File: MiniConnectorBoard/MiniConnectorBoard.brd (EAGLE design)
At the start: 31.1 x 68.6 mm, 4 parts

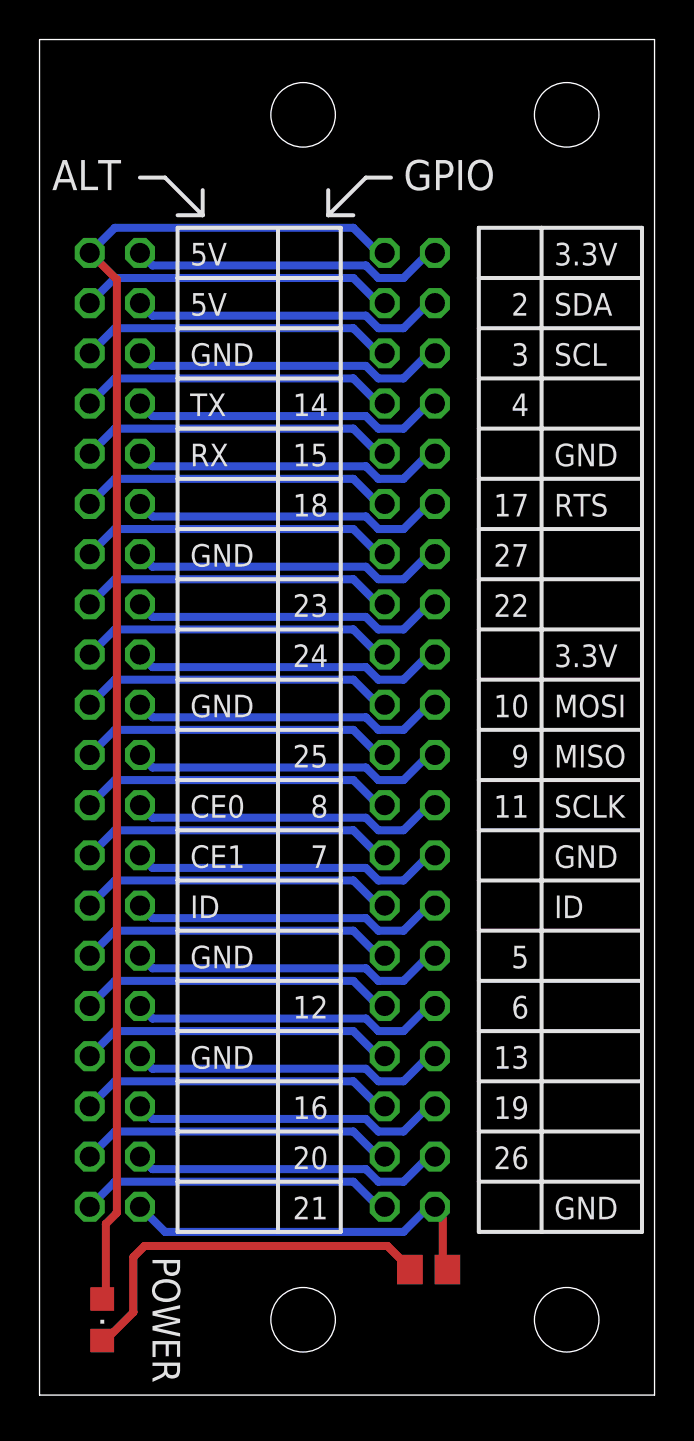
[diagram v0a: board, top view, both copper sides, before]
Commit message: MiniConnectorBoard - first cut
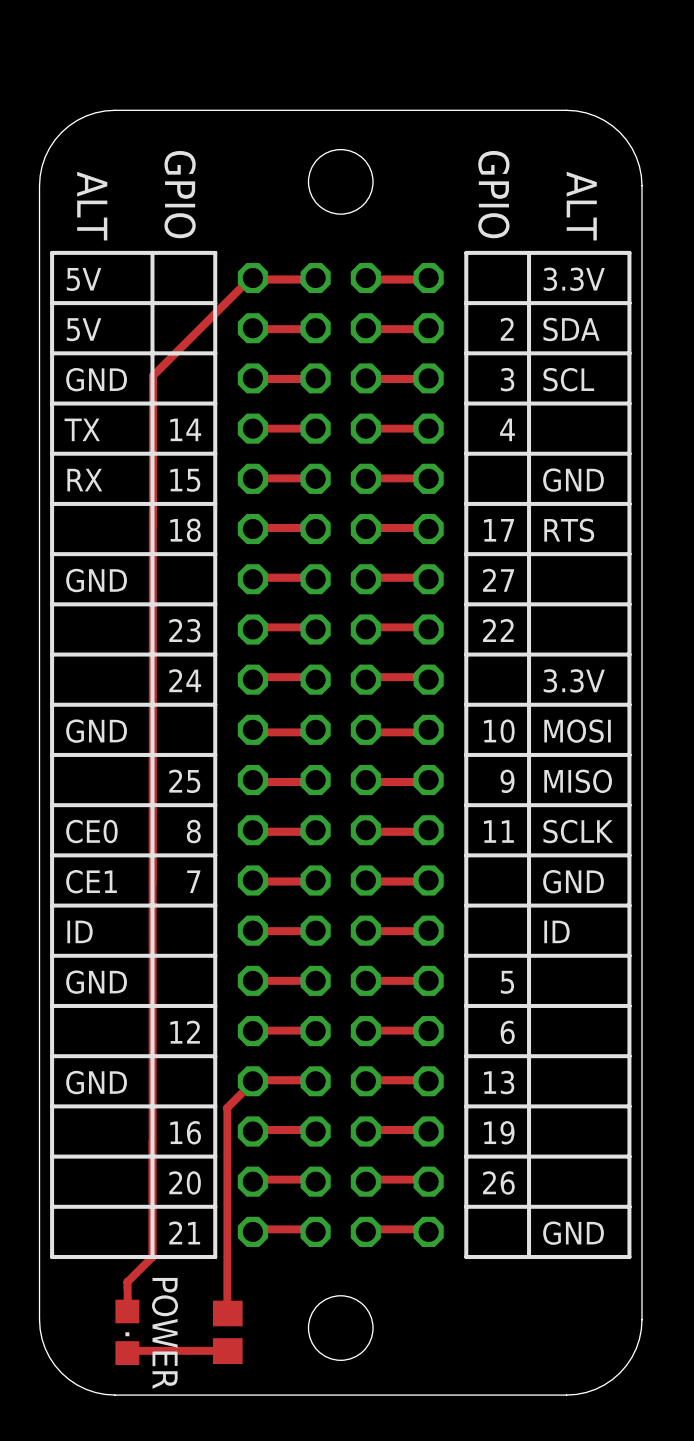
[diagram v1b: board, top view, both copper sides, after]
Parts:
- added JP3: NONE, MiniConnectorBoard:1X20
- JP2: device HeaderConnectorBoard:2X20 -> MiniConnectorBoard:1X20
- moved R1 10.6 mm to (9.53, 3.17), turned to 270 degrees
- moved JP2 8.35 mm to (12.1, 32.4)
- moved JP1 3.72 mm to (15.2, 32.4)
- moved LED1 1.42 mm to (4.45, 3.17)
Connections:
- net 10/MOSI: now also JP3.10; no longer JP2.20
- net 11/CLK: now also JP3.12; no longer JP2.24
- net 12: now also JP2.16; no longer JP2.31
- net 13: now also JP3.17; no longer JP2.34
- net 14/TX: now also JP2.4; no longer JP2.7
- net 15/RX: now also JP2.5; no longer JP2.9
- net 16: now also JP2.18; no longer JP2.35
- net 17/RTS: now also JP3.6; no longer JP2.12
- net 18: now also JP2.6; no longer JP2.11
- net 19: now also JP3.18; no longer JP2.36
- net 2/SDA: now also JP3.2; no longer JP2.4
- net 20: now also JP2.19; no longer JP2.37
- net 21: now also JP2.20; no longer JP2.39
- net 22: now also JP3.8; no longer JP2.16
- net 23: now also JP2.8; no longer JP2.15
- net 24: now also JP2.9; no longer JP2.17
- net 25: now also JP2.11; no longer JP2.21
- net 26: now also JP3.19; no longer JP2.38
- net 27: now also JP3.7; no longer JP2.14
- net 3.3V_1: now also JP3.1; no longer JP2.2
- net 3.3V_2: now also JP3.9; no longer JP2.18
- net 3/SCL: now also JP3.3; no longer JP2.6
- net 4: now also JP3.4; no longer JP2.8
- net 5: now also JP3.15; no longer JP2.30
- net 5V_1: now also JP2.2; no longer JP2.3
- net 6: now also JP3.16; no longer JP2.32
- net 7/CE1: now also JP2.13; no longer JP2.25
- net 8/CE0: now also JP2.12; no longer JP2.23
- net 9/MISO: now also JP3.11; no longer JP2.22
- net GND: now also JP3.5; no longer JP2.10
- net GND2: now also JP3.13; no longer JP2.26
- net GND3: now also JP2.10; no longer JP2.19
- net GND4: now also JP2.7; no longer JP2.13
- net GND5: now also JP2.3; no longer JP2.5
- net GND6: now also JP3.20; no longer JP2.40, R1.1
- net GND7: now also JP2.17, R1.1; no longer JP2.33
- net GND8: now also JP2.15; no longer JP2.29
- net ID1: now also JP3.14; no longer JP2.28
- net ID2: now also JP2.14; no longer JP2.27
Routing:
- net GND6: track 19.5 -> 3.26 mm
- net N$1: track 19.7 -> 5.17 mm
- net 5: track 16.0 -> 3.17 mm
- net 14/TX: track 16.0 -> 3.18 mm
- net 4: track 16.0 -> 3.17 mm
- net GND8: track 16.0 -> 3.18 mm
- net GND: track 16.0 -> 3.18 mm
- net ID1: track 16.0 -> 3.18 mm
- net 6: track 16.0 -> 3.18 mm
- net 3/SCL: track 16.0 -> 3.18 mm
- net 17/RTS: track 16.0 -> 3.19 mm
- net GND2: track 16.0 -> 3.19 mm
- net 13: track 16.0 -> 3.19 mm
- net 2/SDA: track 16.0 -> 3.19 mm
- net 7/CE1: track 16.0 -> 3.24 mm
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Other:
- board size 31.1 x 68.6 mm -> 30.5 x 65 mm
- board text added: "Rev-01a (c) 2016 Ready Set STEM"
- board text removed: "Rev-02a (c) 2016 Ready Set STEM"
